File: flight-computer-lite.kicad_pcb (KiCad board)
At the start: 2 copper layers, 65 x 65 mm, 85 parts, among them J1 USB_C_Receptacle_USB2.0_16P, J2 Micro_SD_Card_Det2, J3 Conn_01x02_Pin, J4 Conn_01x03_Pin, Q1 BSS138, SW1 SW_Push, SW2 SW_Push, U1 RP2040, U10 SAM-M10Q, U11 LM66200DRLR, U2 W25Q32JVZP, U3 ICM-42688-P, U4 BMI088, U5 LIS3MDL, U6 SHT4x, U7 TPS631000DRLR, U8 INA232AIDDFR, U9 MS5611-01BA, Y1 SiT1602BI-22-33E-12.000000E

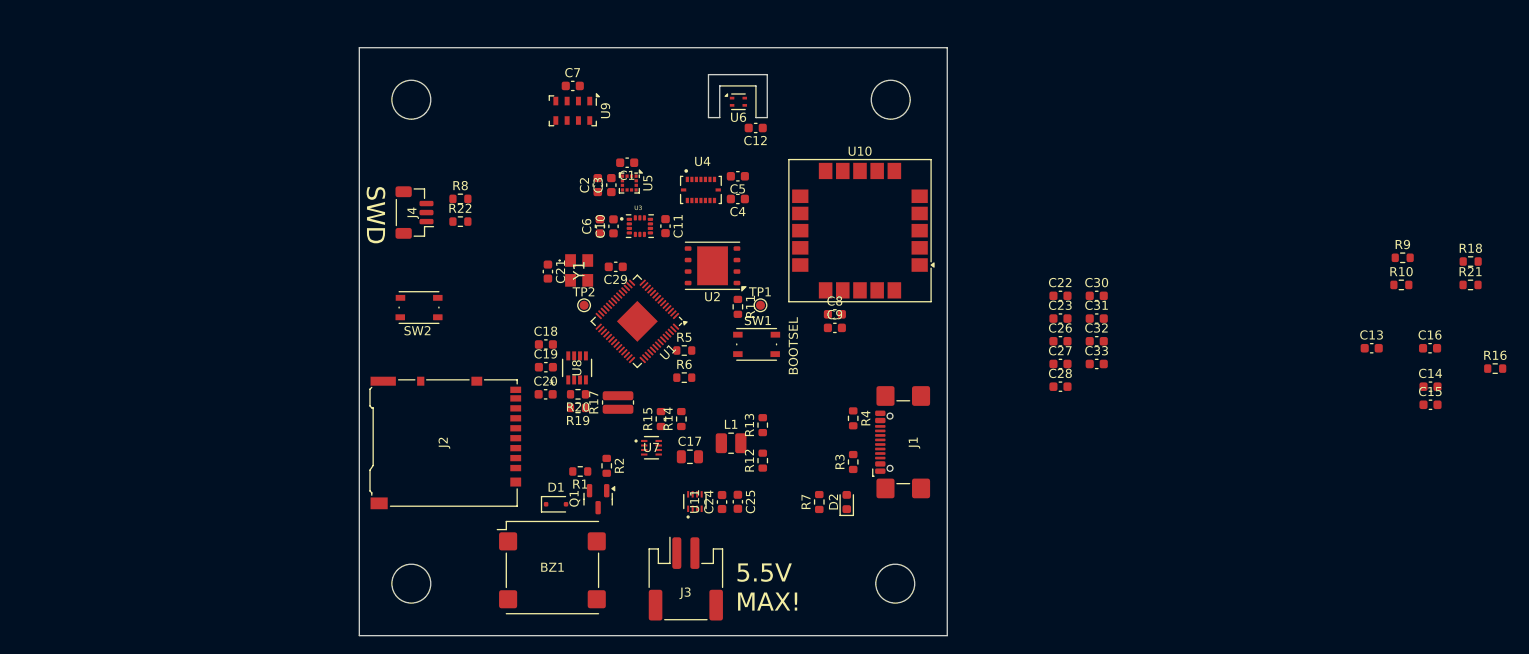
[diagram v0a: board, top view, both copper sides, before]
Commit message: WIP layout/route
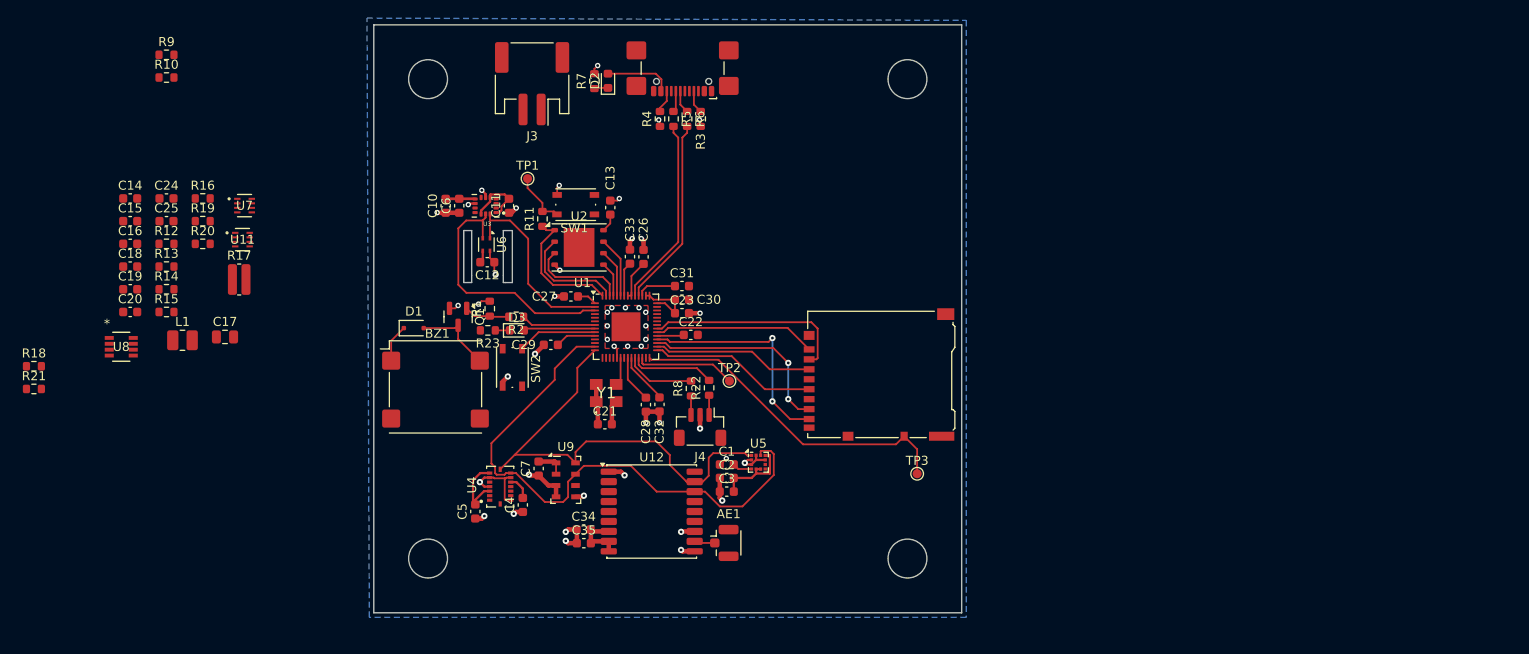
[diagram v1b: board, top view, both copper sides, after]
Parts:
- removed C8: 1u, Capacitor_SMD:C_0603_1608Metric
- removed C9: 0.1u, Capacitor_SMD:C_0603_1608Metric
- removed U10: SAM-M10Q, RF_GPS:ublox_SAM-M8Q
- added AE1: Antenna, Connector_Coaxial:U.FL_Hirose_U.FL-R-SMT-1_Vertical, F.Cu at (166.5, 110.0)
- added C34: 0.1u, Capacitor_SMD:C_0603_1608Metric, F.Cu at (150.9, 108.5)
- added C35: 1u, Capacitor_SMD:C_0603_1608Metric, F.Cu at (151.0, 110.0)
- added D3: LED, LED_SMD:LED_0603_1608Metric, F.Cu at (143.6, 86.5)
- added R23: R, Resistor_SMD:R_0603_1608Metric, F.Cu at (140.4, 86.5)
- added TP3: TestPoint, TestPoint:TestPoint_Pad_D1.0mm, F.Cu at (187.8, 102.4)
- added U12: MAX-M10S, LRI_partlib:ublox_MAX, F.Cu at (158.5, 106.5)
- C30, C31: value 2.2u -> 1u
- R10, R18, R21, R9: value I2C -> 1k
- moved R18 159.3 mm to (90.2, 90.5)
- moved R21 159.2 mm to (90.2, 93.0)
- moved C14 145.3 mm to (100.8, 71.9)
- moved C15 145.2 mm to (100.8, 74.5)
- moved C16 144.2 mm to (100.8, 77.0)
- moved R16 144.1 mm to (108.8, 71.9)
- moved R9 138.5 mm to (104.8, 56.1)
- moved R10 138.4 mm to (104.8, 58.6)
- moved C13 85.6 mm to (153.9, 73.0), turned to 90 degrees
- moved C25 70.4 mm to (104.8, 74.5), turned to 0 degrees
- moved R12 70.1 mm to (104.8, 77.0), turned to 0 degrees
- moved C24 70.0 mm to (104.8, 71.9), turned to 0 degrees
- moved R13 68.2 mm to (104.8, 79.5), turned to 0 degrees
- moved L1 61.7 mm to (106.6, 87.6)
- moved R14 58.7 mm to (104.8, 82.0), turned to 0 degrees
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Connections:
- net /PSU/ST renamed /PSU/POR_ST
- J2 pad 1: unconnected-(J2-DAT2-Pad1) -> /DAT2
- J2 pad 10: /SD_DET -> /CARD_DET
- J2 pad 2: unconnected-(J2-DAT3/CD-Pad2) -> /DAT3/CS
- J2 pad 3: unconnected-(J2-CMD-Pad3) -> /CMD/MOSI
- J2 pad 5: unconnected-(J2-CLK-Pad5) -> /SD_CLK
- J2 pad 7: unconnected-(J2-DAT0-Pad7) -> /DAT0/MISO
- J2 pad 8: unconnected-(J2-DAT1-Pad8) -> /DAT1
- SW2 pad 1: /USR -> /USR_BTN
- U1 pad 13: unconnected-(U1-GPIO10-Pad13) -> /I2C Bus 2/I2C_2_SDA
- U1 pad 14: unconnected-(U1-GPIO11-Pad14) -> /I2C Bus 2/I2C_2_SCL
- U1 pad 16: /USR -> unconnected-(U1-GPIO13-Pad16)
- U1 pad 2: /I2C_1_SDA -> /I2C Bus 1/I2C_1_SDA
- U1 pad 28: unconnected-(U1-GPIO17-Pad28) -> /CARD_DET
- U1 pad 29: unconnected-(U1-GPIO18-Pad29) -> /SD_CLK
- U1 pad 3: /I2C_1_SCL -> /I2C Bus 1/I2C_1_SCL
- U1 pad 30: unconnected-(U1-GPIO19-Pad30) -> /CMD/MOSI
- U1 pad 31: unconnected-(U1-GPIO20-Pad31) -> /DAT0/MISO
- U1 pad 32: unconnected-(U1-GPIO21-Pad32) -> /DAT1
- U1 pad 34: unconnected-(U1-GPIO22-Pad34) -> /DAT2
- U1 pad 35: unconnected-(U1-GPIO23-Pad35) -> /DAT3/CS
- U1 pad 4: /I2C Bus 2/I2C_2_SDA -> unconnected-(U1-GPIO2-Pad4)
- U1 pad 43: unconnected-(U1-ADC_AVDD-Pad43) -> +3V3
- U1 pad 45: +3V3 -> +1V1
- U1 pad 5: /I2C Bus 2/I2C_2_SCL -> unconnected-(U1-GPIO3-Pad5)
- U1 pad 7: unconnected-(U1-GPIO5-Pad7) -> /BUZZER_CTL
- U1 pad 8: unconnected-(U1-GPIO6-Pad8) -> /USR_LED
- U1 pad 9: unconnected-(U1-GPIO7-Pad9) -> /USR_BTN
- U5 pad 1: /I2C Bus 1/I2C_1_SCL -> /I2C Bus 2/I2C_2_SCL
- U5 pad 11: /I2C Bus 1/I2C_1_SDA -> /I2C Bus 2/I2C_2_SDA
- U8 pad 5: /PSU/I2C_1_SCL -> /I2C Bus 1/I2C_1_SCL
- U8 pad 6: /PSU/I2C_1_SDA -> /I2C Bus 1/I2C_1_SDA
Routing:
- net +3V3: track 0.00 -> 78.5 mm
- net GND: track 0.00 -> 66.1 mm, vias 0 -> 47
- net /I2C Bus 2/I2C_2_SDA: track 0.00 -> 62.7 mm
- net /I2C Bus 2/I2C_2_SCL: track 0.00 -> 50.8 mm
- net /CARD_DET: track 0.00 -> 37.2 mm
- net /I2C Bus 1/I2C_1_SCL: track 0.00 -> 28.6 mm
- net /DAT1: track 0.00 -> 24.9 mm, vias 0 -> 2
- net /DAT3/CS: track 0.00 -> 22.6 mm
- net /DAT0/MISO: track 0.00 -> 22.2 mm, vias 0 -> 2
- net /I2C Bus 1/I2C_1_SDA: track 0.00 -> 21.2 mm
- net /CPU_USB_D-: track 0.00 -> 20.9 mm
- net /CPU_USB_D+: track 0.00 -> 20.9 mm
- net /SD_CLK: track 0.00 -> 18.6 mm
- net /DAT2: track 0.00 -> 18.0 mm
- net /CMD/MOSI: track 0.00 -> 17.8 mm
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- added copper zone on B.Cu, net GND
- added copper zone on F.Cu, net GND
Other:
- outline, holes or cut-outs redrawn
- rule pad_to_mask_clearance: 0 -> 0.0508
- board text removed: "5.5V MAX!"
- board text removed: "BOOTSEL"
- board text removed: "SWD"
